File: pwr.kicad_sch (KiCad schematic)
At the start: 6 parts, among them J1 GSB1C4621DSHR

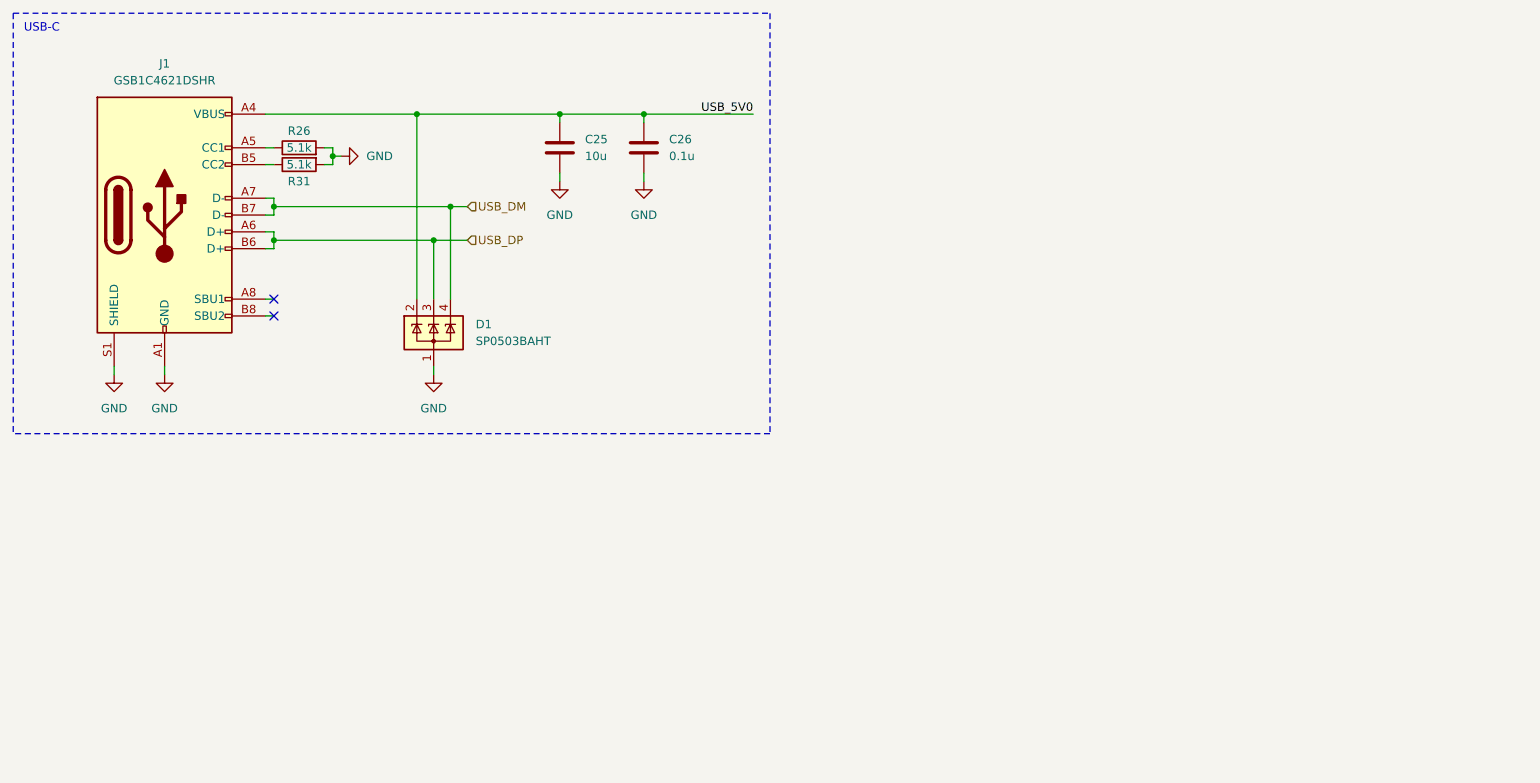
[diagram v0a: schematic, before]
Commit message: sch_0v1 ready for review
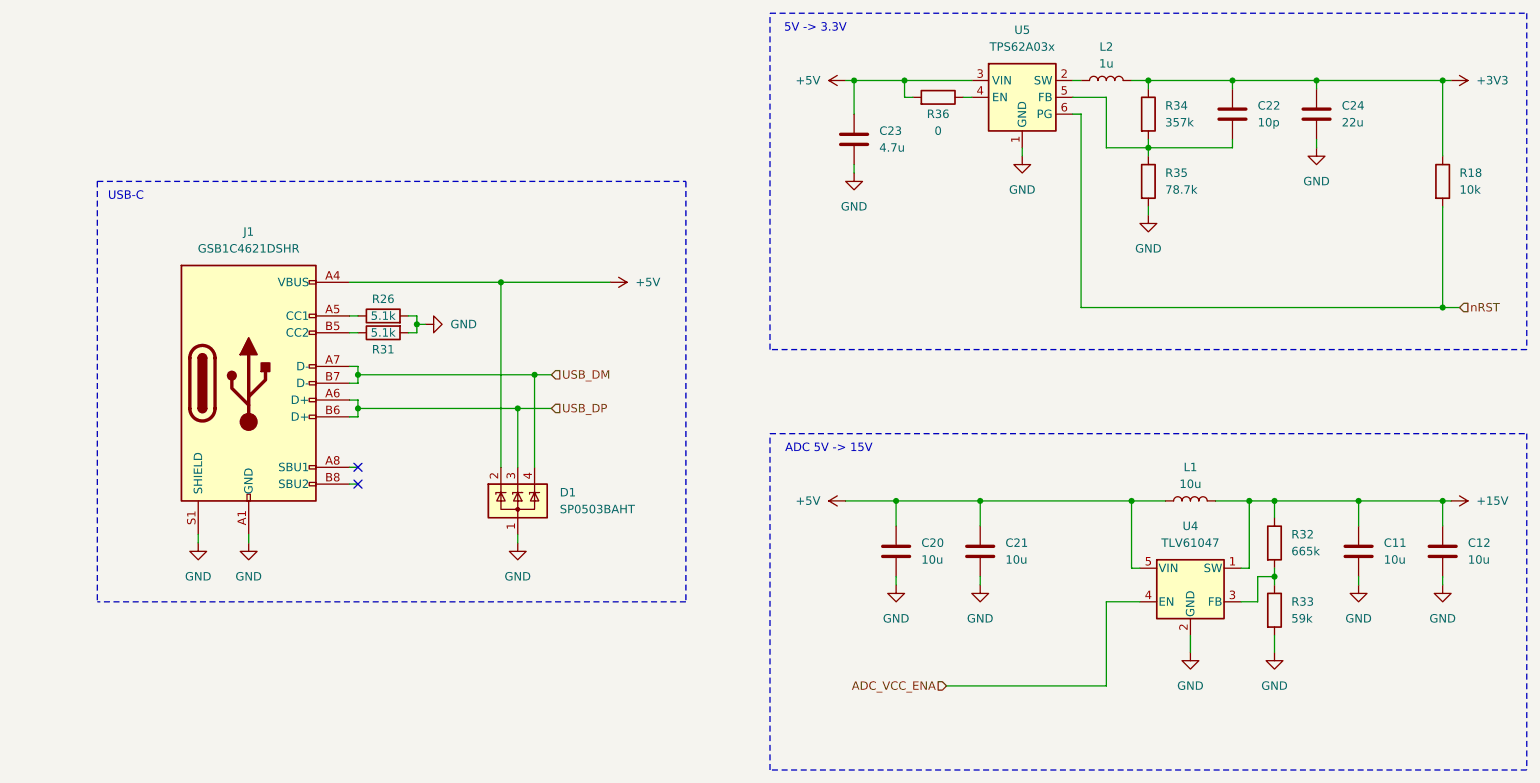
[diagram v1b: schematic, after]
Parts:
- removed C25: 10u, symbol Device:C
- removed C26: 0.1u, symbol Device:C
- added C11, C12, C20, C21: 10u, symbol Device:C
- added C22: 10p, symbol Device:C
- added C23: 4.7u, symbol Device:C
- added C24: 22u, symbol Device:C
- added L1: 10u, symbol Device:L
- added L2: 1u, symbol Device:L
- added R18: 10k, symbol Device:R
- added R32: 665k, symbol Device:R
- added R33: 59k, symbol Device:R
- added R34: 357k, symbol Device:R
- added R35: 78.7k, symbol Device:R
- added R36: 0, symbol Device:R
- added U4: TLV61047, Package_TO_SOT_SMD:SOT-23-5, symbol generated_symbols:TLV61407
- added U5: TPS62A03x, Package_TO_SOT_SMD:SOT-563, symbol generated_symbols:TPS62A03x
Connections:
- net GND: now also C11.2, C12.2, C20.2, C21.2, C23.2, C24.2, R33.2, R35.2, U4.2 (GND), U5.1 (GND)
- net USB_5V0 renamed +5V
- net +5V: now also C20.1, C21.1, C23.1, L1.1, R36.2, U4.5 (VIN), U5.3 (VIN)
- new net: C22.2, R34.2, R35.1, U5.5 (FB)
- new net: R32.2, R33.1, U4.3 (FB)
- new net: L2.1, U5.2 (SW)
- new net: R36.1, U5.4 (EN)
- new net +15V: C11.1, C12.1, L1.2, R32.1, U4.1 (SW)
- new net +3V3: C22.1, C24.1, L2.2, R18.1, R34.1
- new net ADC_VCC_ENA: U4.4 (EN)
- new net nRST: R18.2, U5.6 (PG)
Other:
- note added: "5V -> 3.3V"
- note added: "ADC 5V -> 15V"
- moved on the sheet: D1, J1, R26, R31
